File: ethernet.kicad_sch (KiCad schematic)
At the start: 20 parts, among them U6 RTL8211F-CG

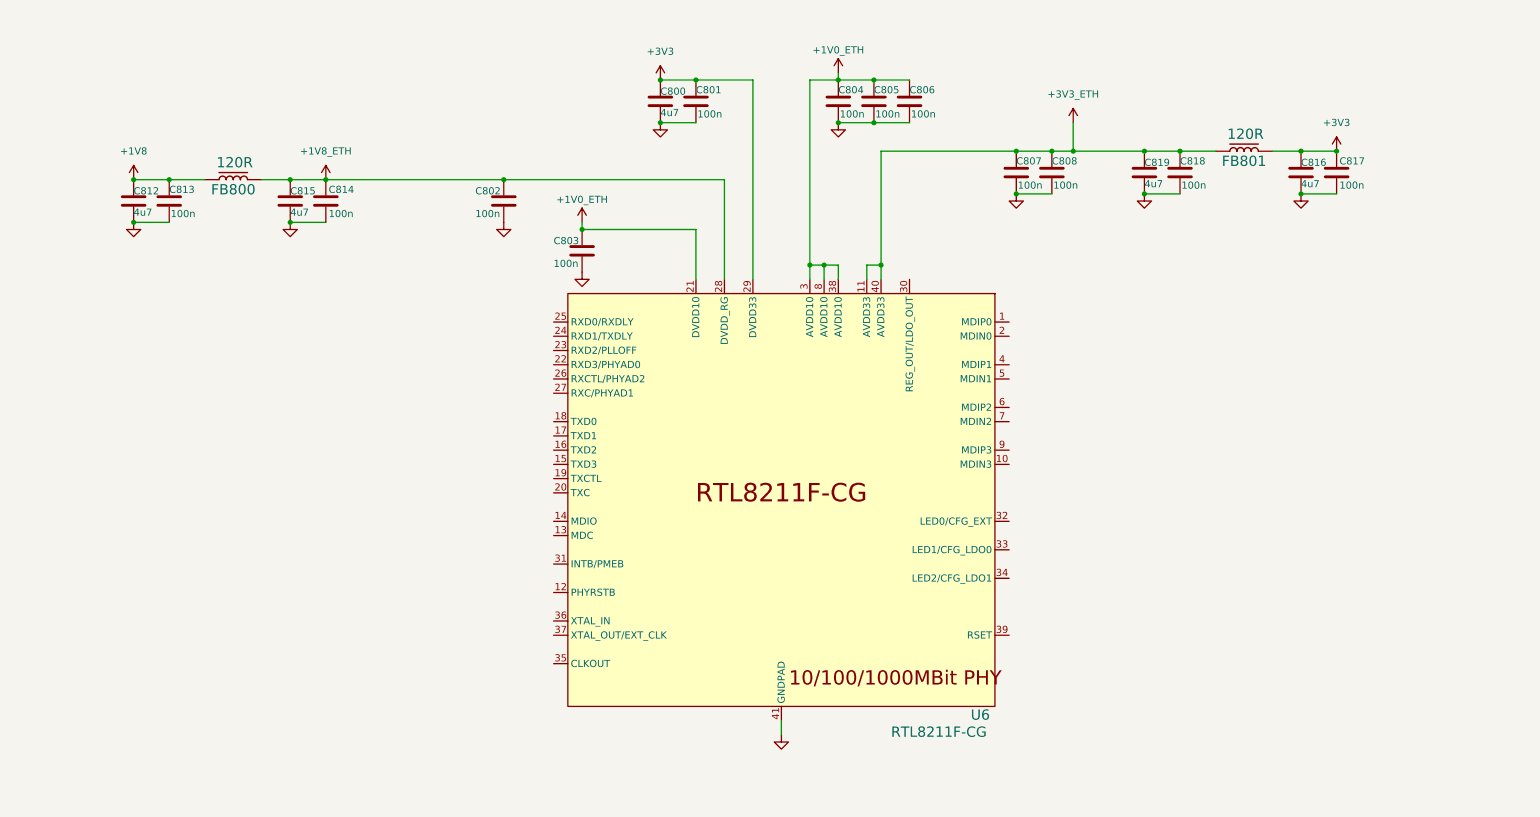
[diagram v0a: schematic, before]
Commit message: sch-eth-usb-updated
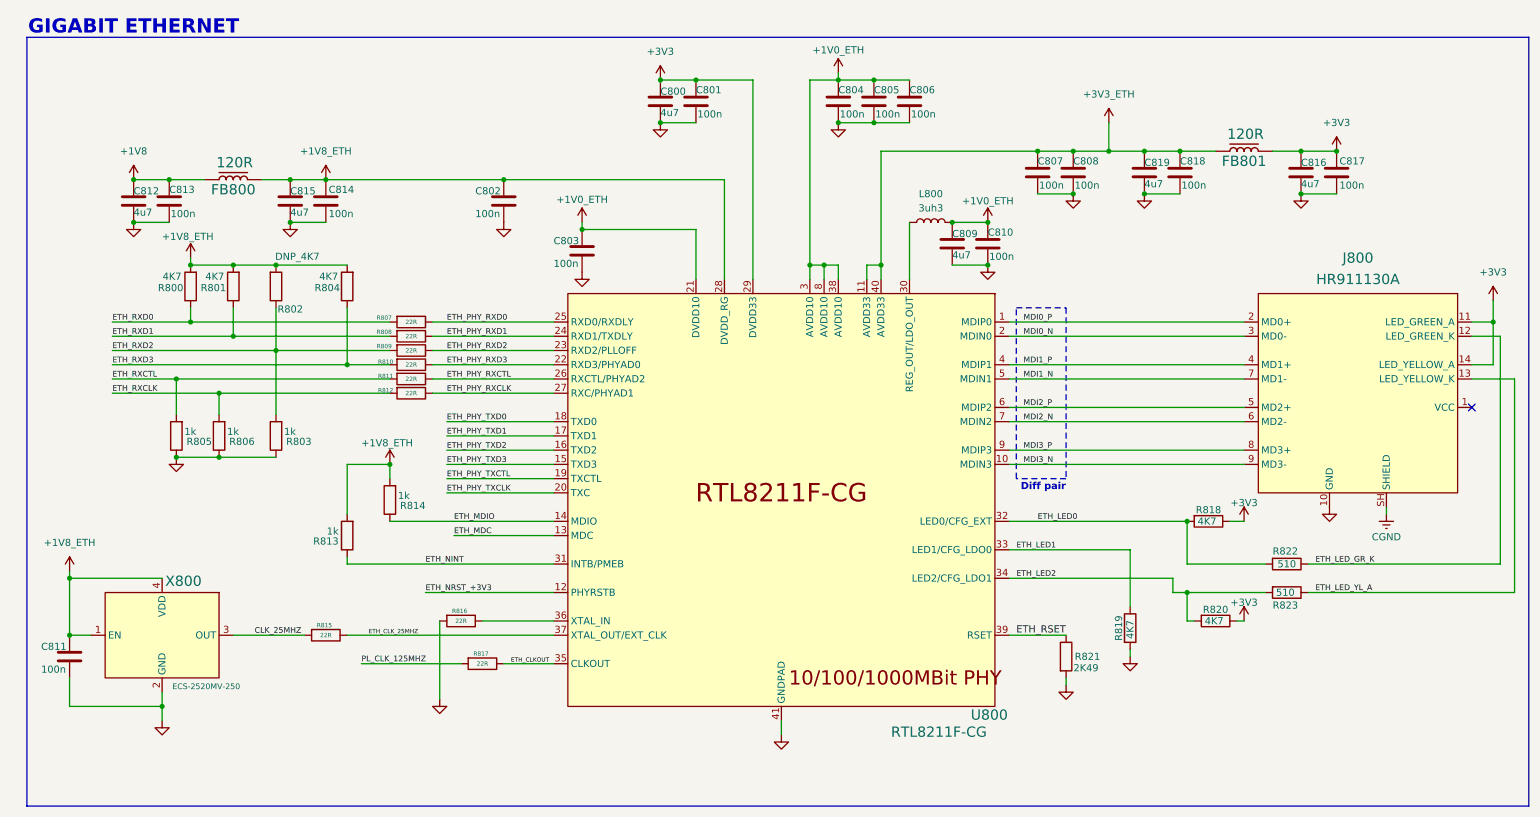
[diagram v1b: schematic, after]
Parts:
- added C809: 4u7, Capacitor_SMD:C_0402_1005Metric, symbol Device:C
- added C810, C811: 100n, Capacitor_SMD:C_0402_1005Metric, symbol Device:C
- added J800: HR911130A, HR911130A, symbol Schematic-Lib-PhilsLab:HR911130A
- added L800: 3uh3, Inductor_SMD:L_0603_1608Metric, symbol Device:L
- added R800, R801, R804, R818, R819, R820: 4K7, Resistor_SMD:R_0402_1005Metric, symbol Device:R
- added R802: DNP_4K7, Resistor_SMD:R_0402_1005Metric, symbol Device:R
- added R803, R805, R806, R813, R814: 1k, Resistor_SMD:R_0402_1005Metric, symbol Device:R
- added R807, R808, R809, R810, R811, R812, R815, R816, R817: 22R, Resistor_SMD:R_0402_1005Metric, symbol Device:R
- added R821: 2K49, Resistor_SMD:R_0402_1005Metric, symbol Device:R
- added R822, R823: 510, Resistor_SMD:R_0402_1005Metric, symbol Device:R
- added X800: ECS-2520MV-250, XTAL_2520, symbol Schematic-Lib-PhilsLab:ECS-2520MV-130-BN-TR
- renumbered U6 to U800
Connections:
- net +1V0_ETH: now also C809.1, C810.1, L800.2
- net +1V8_ETH: now also C811.1, R800.2, R801.2, R802.2, R804.2, R813.2, R814.2, X800.1 (EN), X800.4 (VDD)
- net +3V3: now also J800.11 (LED_GREEN_A), J800.14 (LED_YELLOW_A), R818.1, R820.1
- net GND: now also C809.2, C810.2, C811.2, J800.10 (GND), R803.1, R805.1, R806.1, R816.2, R819.2, R821.2, X800.2 (GND)
- net MDI0_P: now reaches U800.1 (MDIP0)
- net MDI0_P: now also J800.2 (MD0+)
- net MDI3_N: now reaches U800.10 (MDIN3)
- net MDI3_N: now also J800.9 (MD3-)
- net ETH_NRST_+3V3: now reaches U800.12 (PHYRSTB)
- net ETH_MDC: now reaches U800.13 (MDC)
- net ETH_MDIO: now reaches U800.14 (MDIO)
- net ETH_MDIO: now also R814.1
- net ETH_PHY_TXD3: now reaches U800.15 (TXD3)
- net ETH_PHY_TXD2: now reaches U800.16 (TXD2)
- net ETH_PHY_TXD1: now reaches U800.17 (TXD1)
- net ETH_PHY_TXD0: now reaches U800.18 (TXD0)
- net ETH_PHY_TXCTL: now reaches U800.19 (TXCTL)
- net MDI0_N: now reaches U800.2 (MDIN0)
- net MDI0_N: now also J800.3 (MD0-)
- net ETH_PHY_TXCLK: now reaches U800.20 (TXC)
- net ETH_PHY_RXD3: now reaches U800.22 (RXD3/PHYAD0)
- net ETH_PHY_RXD3: now also R810.1
- net ETH_PHY_RXD2: now reaches U800.23 (RXD2/PLLOFF)
- net ETH_PHY_RXD2: now also R809.1
- net ETH_PHY_RXD1: now reaches U800.24 (RXD1/TXDLY)
- net ETH_PHY_RXD1: now also R808.1
- net ETH_PHY_RXD0: now reaches U800.25 (RXD0/RXDLY)
- net ETH_PHY_RXD0: now also R807.1
- net ETH_PHY_RXCTL: now reaches U800.26 (RXCTL/PHYAD2)
- net ETH_PHY_RXCTL: now also R811.1
- net ETH_PHY_RXCLK: now reaches U800.27 (RXC/PHYAD1)
- net ETH_PHY_RXCLK: now also R812.1
- net at U800.30 (REG_OUT/LDO_OUT): now also L800.1
- net ETH_NINT: now reaches U800.31 (INTB/PMEB)
- net ETH_NINT: now also R813.1
- net ETH_LED0: now reaches U800.32 (LED0/CFG_EXT)
- net ETH_LED0: now also R818.2, R822.2
- net ETH_LED1: now reaches U800.33 (LED1/CFG_LDO0)
- net ETH_LED1: now also R819.1
- net ETH_LED2: now reaches U800.34 (LED2/CFG_LDO1)
- net ETH_LED2: now also R820.2, R823.2
- net ETH_CLKOUT: now reaches U800.35 (CLKOUT)
- net ETH_CLKOUT: now also R817.1
- net at U800.36 (XTAL_IN): now also R816.1
- net ETH_CLK_25MHZ: now reaches U800.37 (XTAL_OUT/EXT_CLK)
- net ETH_CLK_25MHZ: now also R815.1
- net ETH_RSET: now reaches U800.39 (RSET)
- net ETH_RSET: now also R821.1
- net MDI1_P: now reaches U800.4 (MDIP1)
- net MDI1_P: now also J800.4 (MD1+)
- net MDI1_N: now reaches U800.5 (MDIN1)
- net MDI1_N: now also J800.7 (MD1-)
- net MDI2_P: now reaches U800.6 (MDIP2)
- net MDI2_P: now also J800.5 (MD2+)
- net MDI2_N: now reaches U800.7 (MDIN2)
- net MDI2_N: now also J800.6 (MD2-)
- net MDI3_P: now reaches U800.9 (MDIP3)
- net MDI3_P: now also J800.8 (MD3+)
- new net CGND: J800.SH (SHIELD)
- new net CLK_25MHZ: R815.2, X800.3 (OUT)
- new net ETH_LED_GR_K: J800.12 (LED_GREEN_K), R822.1
- new net ETH_LED_YL_A: J800.13 (LED_YELLOW_K), R823.1
- new net ETH_RXCLK: R806.2, R812.2
- new net ETH_RXCTL: R805.2, R811.2
- new net ETH_RXD0: R800.1, R807.2
- new net ETH_RXD1: R801.1, R808.2
- new net ETH_RXD2: R802.1, R803.2, R809.2
- new net ETH_RXD3: R804.1, R810.2
- new net PL_CLK_125MHZ: R817.2
- no-connect marks 0 -> 1
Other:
- note added: "Diff pair"
- note added: "GIGABIT ETHERNET"
- moved on the sheet: C807, C808
